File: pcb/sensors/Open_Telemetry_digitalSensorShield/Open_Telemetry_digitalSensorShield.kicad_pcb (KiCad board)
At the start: 4 copper layers, 50.8 x 22.9 mm, 45 parts, among them IC1 L80-M39, J1 73412-0110, J2 Conn_01x12_Female, J3 Conn_01x16_Female, Q1 BC846BPN, U1 BME280, U2 MPU-9250

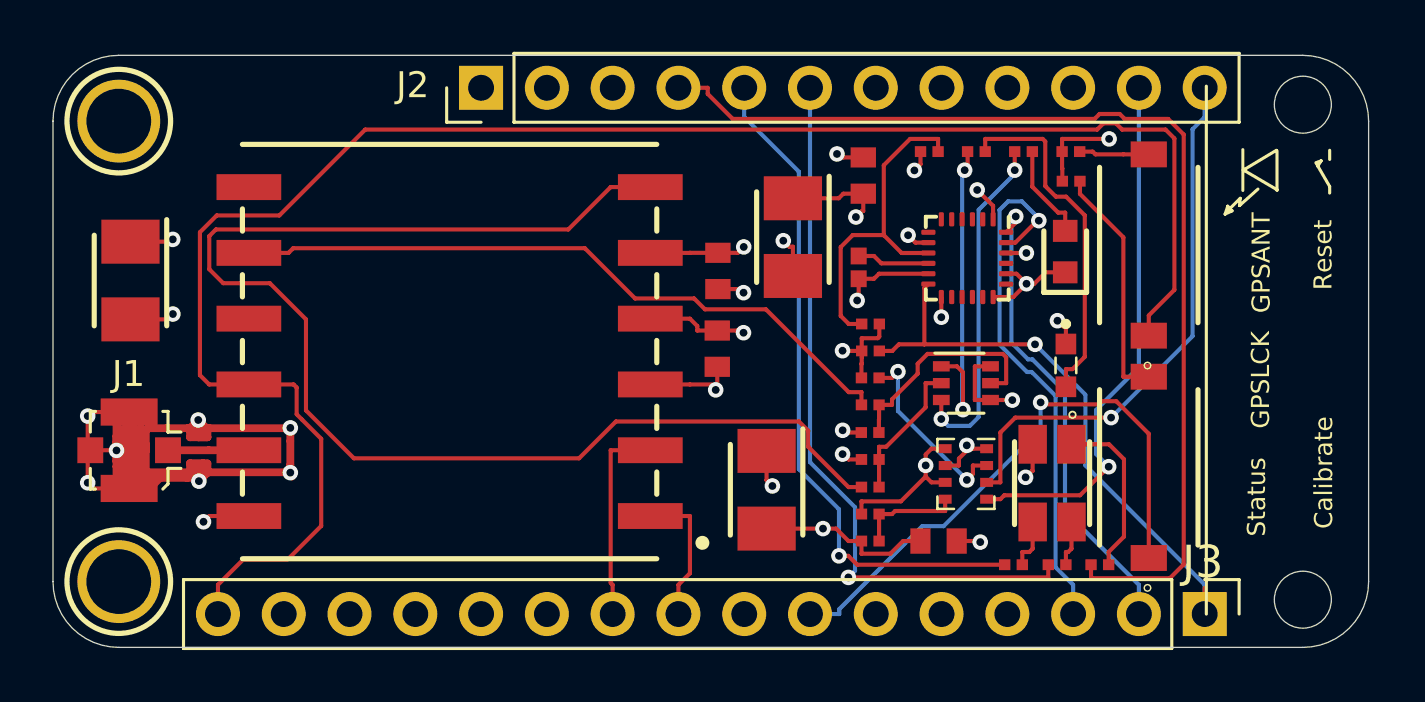
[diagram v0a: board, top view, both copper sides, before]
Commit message: 2'nd internal review
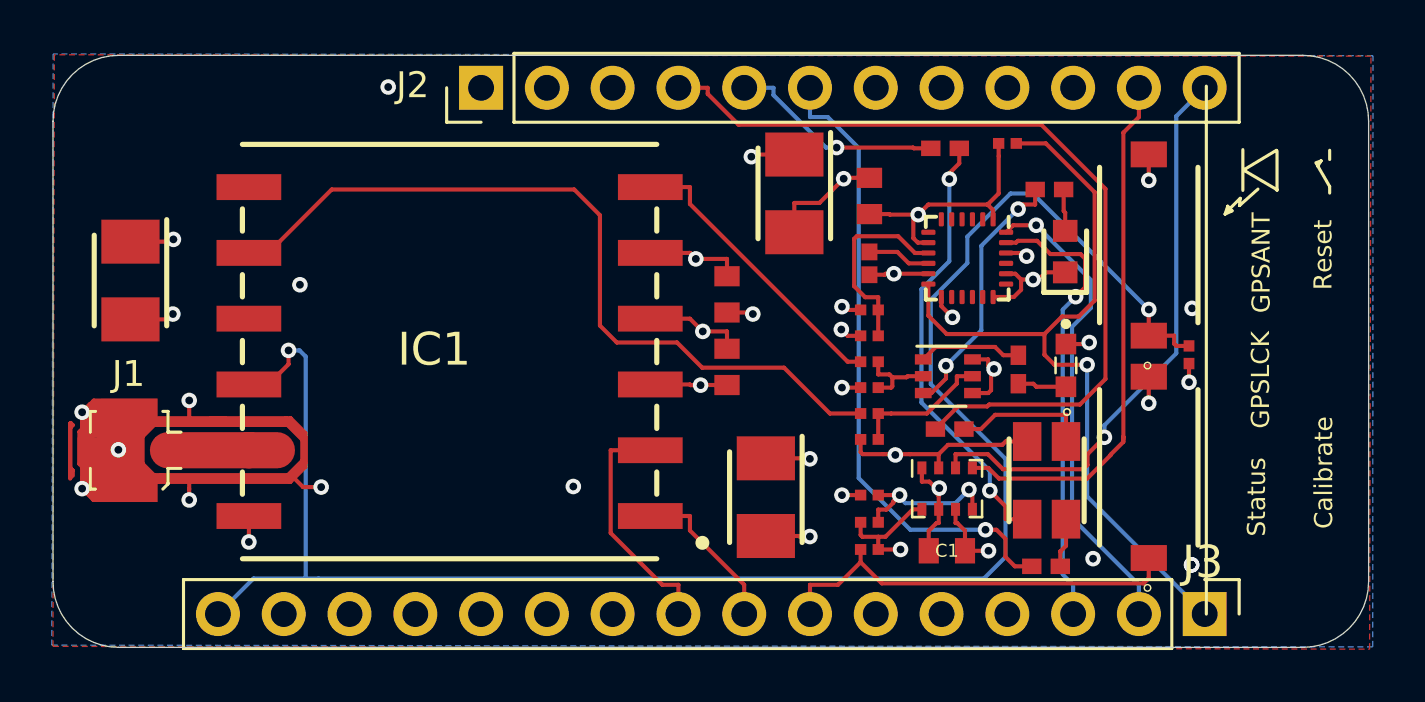
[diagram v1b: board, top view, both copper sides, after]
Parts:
- removed @HOLE0, @HOLE1: , 
- removed D1: ASMB-MTB1-0A3A2, Open_Telemetry:AVAGO_PLCC4
- removed G***: LOGO, Open_Telemetry:BLUETOOTH
- removed G***: LOGO, Open_Telemetry:OpenFlyTelemetry
- removed G***: LOGO, Open_Telemetry:WIFI
- removed G***: LOGO, Open_Telemetry:GPS
- removed R17: 1k, RESC0603X26N
- removed U$31, U$32: MOUNTINGHOLE2.5, Adafruit HUZZAH32 ESP32 Feather:MOUNTINGHOLE_2.5_PLATED
- added LED3: , Open_Telemetry:AVAGO_PLCC4, F.Cu at (252.3, 148.4)
- C1, C2, C3, C4: footprint CAPC1608X87N -> Open_Telemetry:CAPC1608X87N
- C5: footprint CAPC1005X55N -> Open_Telemetry:CAPC1005X55N
- IC1: footprint L80-M39 -> Open_Telemetry:L80-M39
- J1: value 73412-0110 -> Ext GPS antenna connector
- J2: value Conn_01x12_Female -> PinHeader_01x12
- J3: value Conn_01x16_Female -> PinHeader_01x16
- LED1: value ExtAnt -> EXT ANT
- R1, R9: footprint RESC0603X26N -> Open_Telemetry:RESC0603X26N
- R10: value 10k -> 62; footprint RESC0603X26N -> Open_Telemetry:RESC1005X40N
- R11, R12, R13: value 1k -> 62; footprint RESC0603X26N -> Open_Telemetry:RESC1005X40N
- R14: value 1k -> 130; footprint RESC0603X26N -> Open_Telemetry:RESC1005X40N
- R15, R16: value 1k -> 10k; footprint RESC0603X26N -> Open_Telemetry:RESC0603X26N
- R2: value 10k -> 1k; footprint RESC0603X26N -> Open_Telemetry:RESC0603X26N
- R3: value 1k -> 100k; footprint RESC0603X26N -> Open_Telemetry:RESC0603X26N
- R4: value 100k -> NULL
- R5: value NULL -> 100k; footprint RESC0603X26N -> Open_Telemetry:RESC0603X26N
- R6: value 100k -> 1k; footprint RESC0603X26N -> Open_Telemetry:RESC0603X26N
- R7: value 1k -> NULL
- R8: value NULL -> 10k
- moved R16 17.2 mm to (245.5, 151.1)
- moved R10 9.30 mm to (252.4, 137.2)
- moved R15 8.81 mm to (257.8, 143.5), turned to 90 degrees
- moved R11 8.42 mm to (251.2, 144.1), turned to 270 degrees
- moved R14 6.68 mm to (248.6, 146.4)
- moved R5 3.92 mm to (245.5, 146.8), turned to 0 degrees
- moved R3 3.84 mm to (245.5, 144.8)
- moved R9 3.03 mm to (250.8, 135.4), turned to 0 degrees
- moved R7 2.67 mm to (245.5, 142.8)
- moved C7 1.69 mm to (242.6, 137.3)
- moved R4 1.38 mm to (245.5, 148.9)
- moved R13 1.26 mm to (252.3, 151.7)
- moved R12 1.22 mm to (248.4, 135.6)
- moved C3 0.97 mm to (240.0, 141.2)
- moved U1 0.92 mm to (248.5, 148.7), turned to 0 degrees
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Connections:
- IC1 pad 7: Net-(IC1-Pad7) -> (no net)
- IC1 pad 9: Net-(IC1-Pad9) -> (no net)
- J2 pad 1: Net-(J2-Pad1) -> (no net)
- J2 pad 10: Net-(J2-Pad10) -> (no net)
- J2 pad 2: Net-(J2-Pad2) -> (no net)
- J2 pad 3: Net-(J2-Pad3) -> (no net)
- J2 pad 7: Net-(J2-Pad7) -> (no net)
- J2 pad 8: Net-(J2-Pad8) -> (no net)
- J2 pad 9: Net-(J2-Pad9) -> (no net)
- J3 pad 10: UART_1_CLIENT_TXD -> (no net)
- J3 pad 11: Net-(J3-Pad11) -> (no net)
- J3 pad 12: Net-(J3-Pad12) -> (no net)
- J3 pad 14: Net-(J3-Pad14) -> (no net)
- J3 pad 4: Net-(J3-Pad4) -> (no net)
- J3 pad 5: Net-(J3-Pad5) -> (no net)
- J3 pad 6: Net-(J3-Pad6) -> (no net)
- J3 pad 8: Net-(J3-Pad8) -> UART_1_CLIENT_RXD
- J3 pad 9: UART_1_CLIENT_RXD -> UART_1_CLIENT_TXD
- R10 pad 1: +3V3 -> EXT_ANT
- R10 pad 2: INT_0 -> Net-(LED1-Pad2)
- R11 pad 1: EXT_ANT -> SAT_LOCK
- R11 pad 2: Net-(LED1-Pad2) -> Net-(LED2-Pad2)
- R12 pad 1: SAT_LOCK -> BLUE_LED
- R12 pad 2: Net-(LED2-Pad2) -> Net-(LED3-Pad3)
- R13 pad 1: BLUE_LED -> GREEN_LED
- R14 pad 1: GREEN_LED -> RED_LED
- R15 pad 1: RED_LED -> +3V3
- R15 pad 2: Net-(D1-Pad1) -> RESET
- R16 pad 1: Net-(R16-Pad1) -> +3V3
- R16 pad 2: GND -> CALIB
- R2 pad 1: Net-(R2-Pad1) -> Net-(IC1-Pad6)
- R2 pad 2: +3V3 -> Net-(Q1-Pad2)
- R3 pad 1: Net-(IC1-Pad6) -> GND
- R4 pad 2: Net-(Q1-Pad2) -> Net-(R1-Pad2)
- R5 pad 1: Net-(R1-Pad2) -> +3V3
- R5 pad 2: GND -> Net-(Q1-Pad5)
- R6 pad 1: +3V3 -> Net-(IC1-Pad8)
- R7 pad 1: Net-(IC1-Pad8) -> +3V3
- R7 pad 2: Net-(Q1-Pad5) -> Net-(R7-Pad2)
- R8 pad 1: +3V3 -> Net-(R7-Pad2)
- R8 pad 2: Net-(R8-Pad2) -> GND
- R9 pad 1: Net-(R8-Pad2) -> +3V3
- R9 pad 2: GND -> INT_0
- S1 pad 2: Net-(R16-Pad1) -> GND
- S2 pad 2: Net-(R17-Pad1) -> GND
- U1 pad 2: Net-(R2-Pad1) -> +3V3
- U2 pad 21: Net-(U2-Pad21) -> (no net)
- U2 pad 7: Net-(U2-Pad7) -> (no net)
- U2 pad 9: Net-(R8-Pad2) -> Net-(R7-Pad2)
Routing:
- net GND: track 86.3 -> 169.1 mm, vias 21 -> 28
- net Net-(IC1-Pad6): track 51.4 -> 11.3 mm
- net BLUE_LED: track 26.1 -> 8.34 mm
- net Net-(LED3-Pad3): track 0.00 -> 17.1 mm, vias 0 -> 2
- net Net-(R8-Pad2): track 13.2 -> 0.00 mm
- net Net-(LED2-Pad2): track 13.6 -> 1.88 mm
- net Net-(R17-Pad1): track 9.22 -> 0.00 mm
- net +3V3: track 34.3 -> 43.4 mm, vias 15 -> 14
- net RED_LED: track 41.5 -> 32.9 mm
- net SAT_LOCK: track 12.4 -> 4.00 mm, vias 2 -> 0
- net INT_0: track 22.6 -> 30.6 mm
- net Net-(R7-Pad2): track 0.00 -> 7.60 mm
- net Net-(R2-Pad1): track 7.30 -> 0.00 mm, vias 2 -> 0
- net Net-(D1-Pad1): track 6.58 -> 0.00 mm
- net (no net): track 0.00 -> 6.39 mm
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- added copper zone on B.Cu, net GND
- added copper zone on F.Cu, net GND
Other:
- board text added: "Coplanar wawe guide @ 1.5 GHz: Z =(Nom, Max, Min): 49.3 Ohm, X,Y Attenuation (Nom):<2 mdB , H: 0.11 mm (+/- 10%) T: 0.035 mm (+/- 10%) W: 1.4 mm (+/- 10%) S: 0.16 mm (+/- 10%) L: 2 mm (See https://www.pcbway.com/blog/Engineering_Technical/stackup___pcbway.html)"
- board text added: "KeepOut Signals"
- board text removed: "Z=50 Ohms @ 1.5 GHz"
